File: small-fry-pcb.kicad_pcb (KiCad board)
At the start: 2 copper layers, 140 parts, among them U1 Pico

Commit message: fixed rows, generated gerbers
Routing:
- net row2: track 289.8 -> 356.4 mm
- net row0: track 289.2 -> 344.6 mm
- net row1: track 308.5 -> 361.3 mm
- net row3: track 309.3 -> 354.2 mm
- net row4: track 370.1 -> 412.3 mm
- net col14: track 275.7 -> 245.9 mm
- net col6: track 102.0 -> 111.2 mm
- net col13: track 232.5 -> 225.3 mm
- net col0: track 208.6 -> 209.8 mm
- net col1: track 185.8 -> 186.4 mm
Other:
- board outline added: 302 x 150.5 mm

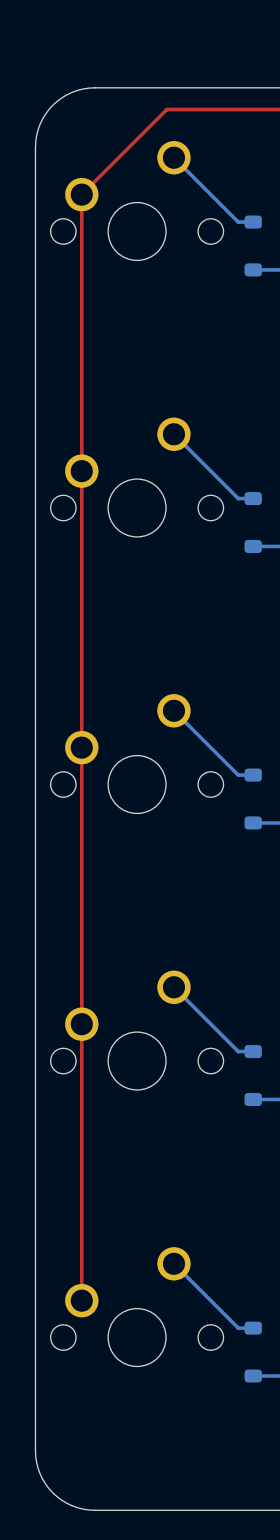
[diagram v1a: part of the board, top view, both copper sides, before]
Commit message: updated edge cuts and gerbers
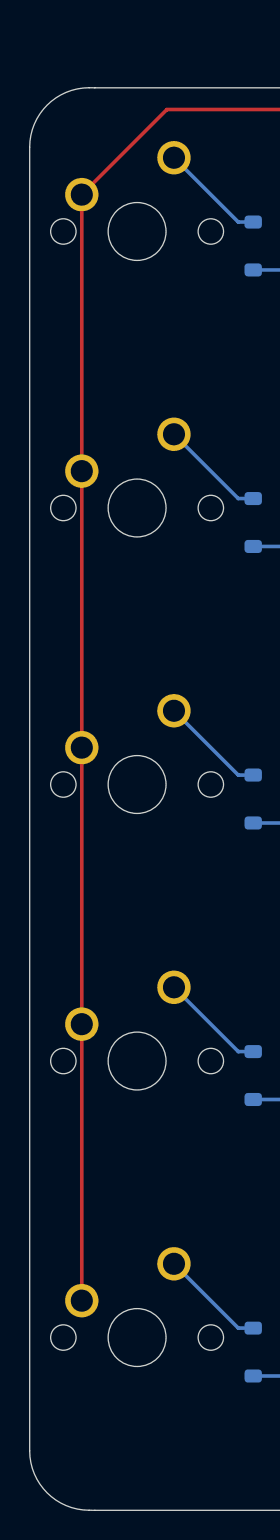
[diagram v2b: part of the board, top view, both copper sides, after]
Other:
- board size 302 x 150.5 mm -> 302.4 x 150.5 mm
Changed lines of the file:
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@@
 	)
 	(gr_line
+		(start 59.09721 167.902801)
+		(end 58.69721 167.897199)
+		(stroke
+			(width 0.09)
+			(type default)
+		)
+		(layer "Edge.Cuts")
+	)
+	(gr_line
 		(start 234.094381 38.837633)
 		(end 206.646664 67.170761)
@@
 	(gr_curve
 		(pts
-			(xy 55 74) (xy 55.000003 71.737181) (xy 56.83438 69.902804) (xy 59.097199 69.902801)
+			(xy 54.6 73.994398) (xy 54.600003 71.731579) (xy 56.43438 69.897202) (xy 58.697199 69.897199)
 		)
 		(stroke
@@
 	(gr_curve
 		(pts
-			(xy 59.09721 167.902801) (xy 56.834387 167.902804) (xy 55.000003 166.068425) (xy 55 163.805602)
+			(xy 58.69721 167.897199) (xy 56.434387 167.897202) (xy 54.600003 166.062823) (xy 54.6 163.8)
 		)
 		(stroke
@@
 		(layer "Edge.Cuts")
 	)
+	(gr_line
+		(start 58.697199 69.897199)
+		(end 59.097199 69.902801)
+		(stroke
+			(width 0.09)
+			(type default)
+		)
+		(layer "Edge.Cuts")
+	)
 	(gr_curve
 		(pts
@@
 	)
 	(gr_line
-		(start 55 163.805602)
-		(end 55 74)
+		(start 54.6 163.8)
+		(end 54.6 73.994398)
 		(stroke
 			(width 0.09)
@@
 	)
 	(group ""
-		(members "26c26e27-6fec-42f9-b5c8-280a722c85c2" "2bdea3e4-563b-40fc-ba2c-ddca74726bf5"
-			"2d6582af-61f5-41ea-8b73-c3fcb968f938" "3613d8ba-32d9-45e9-bf0c-ec0e0fa1bda8"
-			"3f4f9ec1-a3ce-4158-a744-8095b46c3d4f" "42da699c-ed2c-4328-b337-f03ce0245a91"
-			"447c9050-7327-4e40-aa64-af5bbe6642df" "5733d4cc-39a8-49f4-a6bb-032b0f2a0bc1"
-			"578ed080-3792-41c4-9cf0-2628a710686f" "5cf7882a-37bc-4b9d-b738-74cfd924160d"
-			"6aeb5ab6-d3ed-4afd-97d6-2554ad2ac626" "8225f5e9-9778-4593-b414-08246cee0c1e"
-			"83e24ad6-6d31-4f97-add8-d28cdc87d066" "83fec8d0-88fa-47c8-b886-c68763e5efec"
-			"864a073e-e714-4970-a73f-19db9ff1e852" "8e0ae9cc-93b3-44fe-978b-fd3007d24fb7"
-			"91c2bba4-8888-477c-a7cb-b22b75063a7f" "adbd8d92-6597-45da-87a3-4aac6f981cbe"
-			"b910e4a4-1530-4757-a29a-32451da346ff" "c2d9c6d8-4b53-4a71-a272-9ce6d3071683"
-			"cd6f6f85-bf39-421c-b5a1-c768b6ce2a16" "cdb889b8-e4ca-4e48-9e30-0577060eb109"
-			"cf7e58b7-b8d8-405c-b76f-86aabd42e1f5" "dfcc4407-b14d-4c7e-9da9-9e270c260b1b"
+		(members "1b36e1cd-dde7-4b96-9503-0baff936192d" "26c26e27-6fec-42f9-b5c8-280a722c85c2"
+			"2bdea3e4-563b-40fc-ba2c-ddca74726bf5" "2d6582af-61f5-41ea-8b73-c3fcb968f938"
+			"3613d8ba-32d9-45e9-bf0c-ec0e0fa1bda8" "3f4f9ec1-a3ce-4158-a744-8095b46c3d4f"
+			"42da699c-ed2c-4328-b337-f03ce0245a91" "447c9050-7327-4e40-aa64-af5bbe6642df"
+			"5733d4cc-39a8-49f4-a6bb-032b0f2a0bc1" "578ed080-3792-41c4-9cf0-2628a710686f"
+			"5cf7882a-37bc-4b9d-b738-74cfd924160d" "6aeb5ab6-d3ed-4afd-97d6-2554ad2ac626"
+			"8225f5e9-9778-4593-b414-08246cee0c1e" "83e24ad6-6d31-4f97-add8-d28cdc87d066"
+			"83fec8d0-88fa-47c8-b886-c68763e5efec" "864a073e-e714-4970-a73f-19db9ff1e852"
+			"8e0ae9cc-93b3-44fe-978b-fd3007d24fb7" "91c2bba4-8888-477c-a7cb-b22b75063a7f"
+			"adbd8d92-6597-45da-87a3-4aac6f981cbe" "b910e4a4-1530-4757-a29a-32451da346ff"
+			"c2d9c6d8-4b53-4a71-a272-9ce6d3071683" "cd6f6f85-bf39-421c-b5a1-c768b6ce2a16"
+			"cdb889b8-e4ca-4e48-9e30-0577060eb109" "cf7e58b7-b8d8-405c-b76f-86aabd42e1f5"
+			"d45fbdca-ec72-4254-94fe-37604172e439" "dfcc4407-b14d-4c7e-9da9-9e270c260b1b"
 			"f5db2ea6-dfe0-4bf8-b0e8-b5d1a5e7b0f1" "f6da7a7e-e1b3-462d-b275-e868410ca723"
 			"f81ce07c-2d5b-4355-b52d-880095b1a4f7"
